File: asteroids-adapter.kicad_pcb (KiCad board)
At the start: 2 copper layers, 88 x 90.2 mm, 16 parts, among them J1 Asteroids PCB connector, J2 Asteroids harness connector, U1 TL074

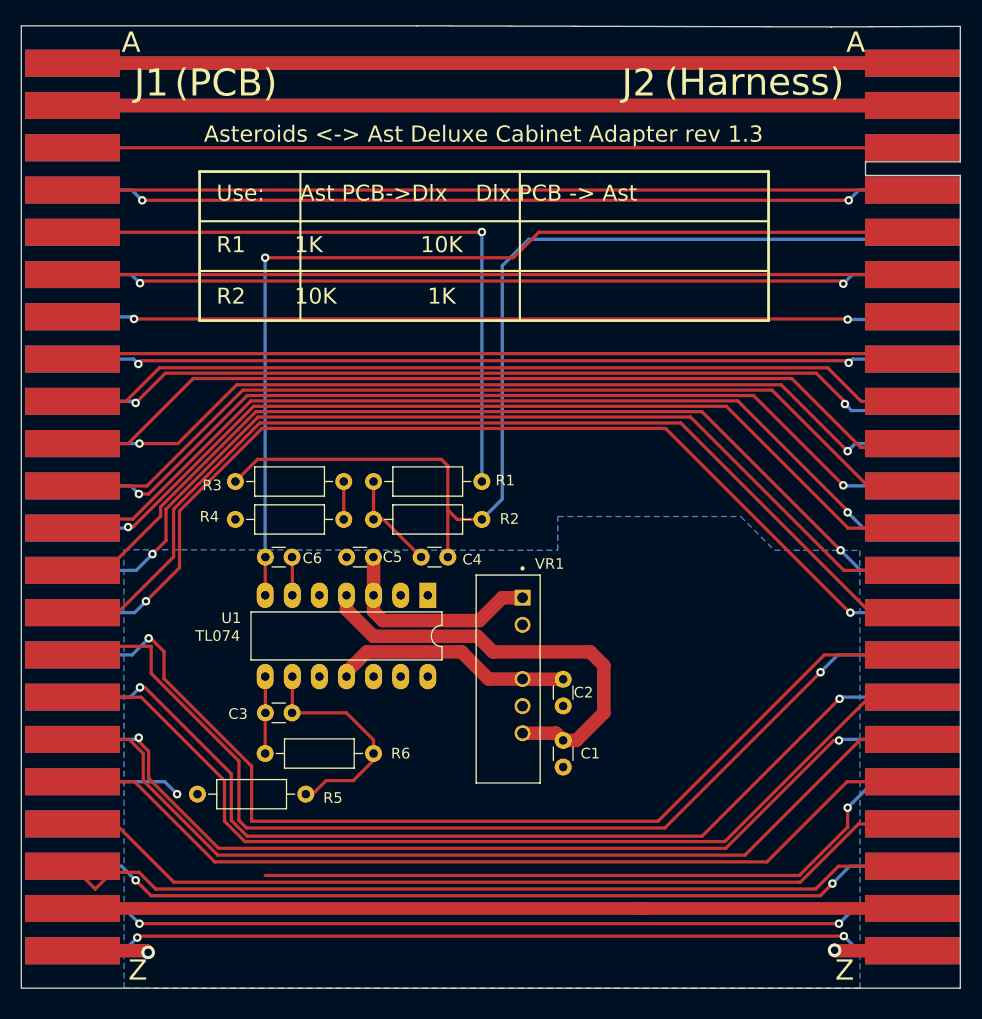
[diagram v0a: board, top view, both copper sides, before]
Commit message: squashed PCB
Still need to clean up PCB outline and re-route
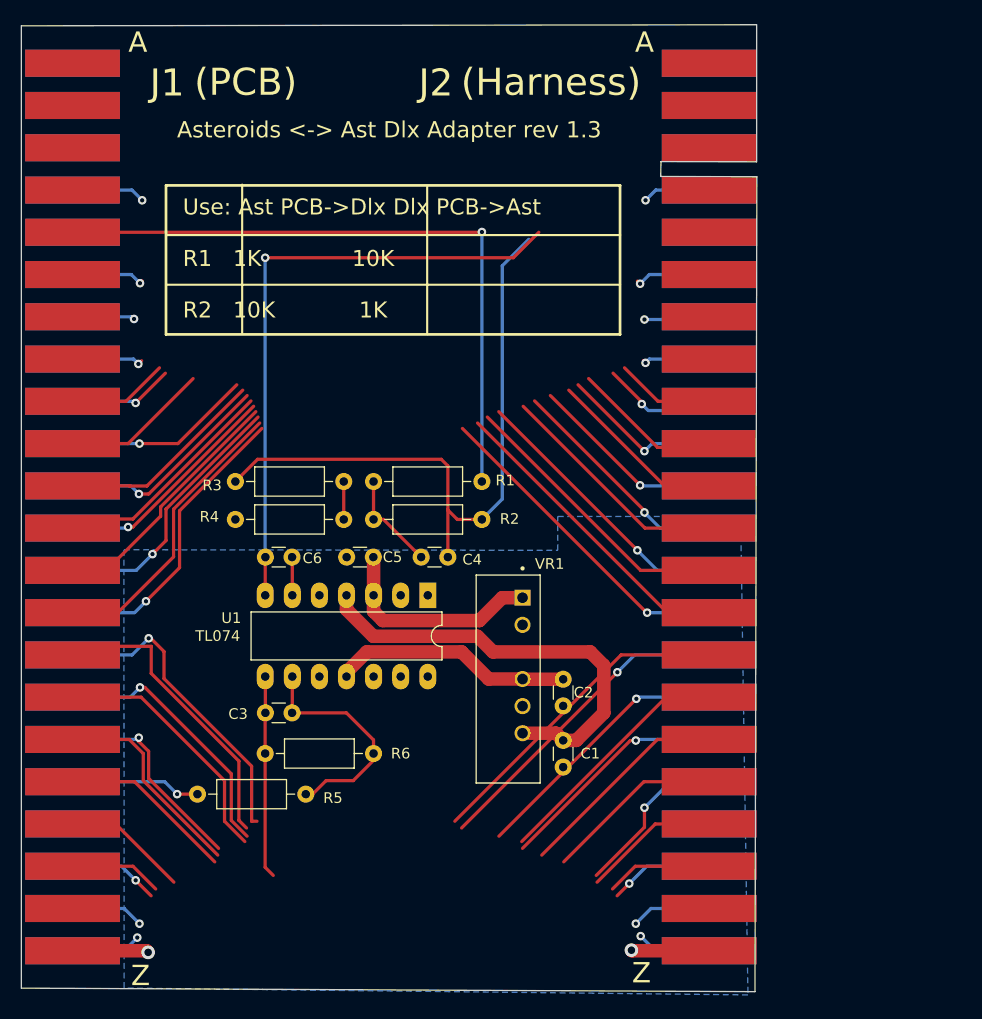
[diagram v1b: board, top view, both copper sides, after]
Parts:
- moved J2 19.1 mm to (167.2, 55.9)
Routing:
- net +5V: track 99.1 -> 20.4 mm
- net Net-(J1-PadF): track 78.7 -> 0.00 mm
- net Net-(J1-PadD): track 78.7 -> 0.00 mm
- net Net-(J1-PadC): track 78.7 -> 0.00 mm
- net Net-(J1-PadB): track 78.7 -> 0.00 mm
- net Net-(J1-PadA): track 78.7 -> 0.00 mm
- net Net-(J1-Pad2): track 78.7 -> 0.00 mm
- net Net-(J1-Pad1): track 78.7 -> 0.00 mm
- net Net-(J1-PadJ): track 79.2 -> 1.44 mm
- net Net-(J1-Pad7): track 79.0 -> 12.1 mm
- net Net-(J1-Pad4): track 79.5 -> 13.3 mm
- net Net-(J1-Pad22): track 79.9 -> 13.8 mm
- net Net-(J1-Pad8): track 79.3 -> 13.2 mm
- net Net-(J1-Pad21): track 79.9 -> 14.3 mm
- net Net-(J1-Pad6): track 79.6 -> 14.1 mm
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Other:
- board size 88 x 90.2 mm -> 69 x 90.7 mm
- board text added: "Asteroids <-> Ast Dlx Adapter rev 1.3"
- board text added: "Use: Ast PCB->Dlx Dlx PCB->Ast R1 1K 10K R2 10K 1K"
- board text removed: "Asteroids <-> Ast Deluxe Cabinet Adapter rev 1.3"
- board text removed: "Use: Ast PCB->Dlx Dlx PCB -> Ast R1 1K 10K R2 10K 1K"
